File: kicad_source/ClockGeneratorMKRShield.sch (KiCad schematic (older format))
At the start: 3 parts, among them CN1 ARDUINO_MKR

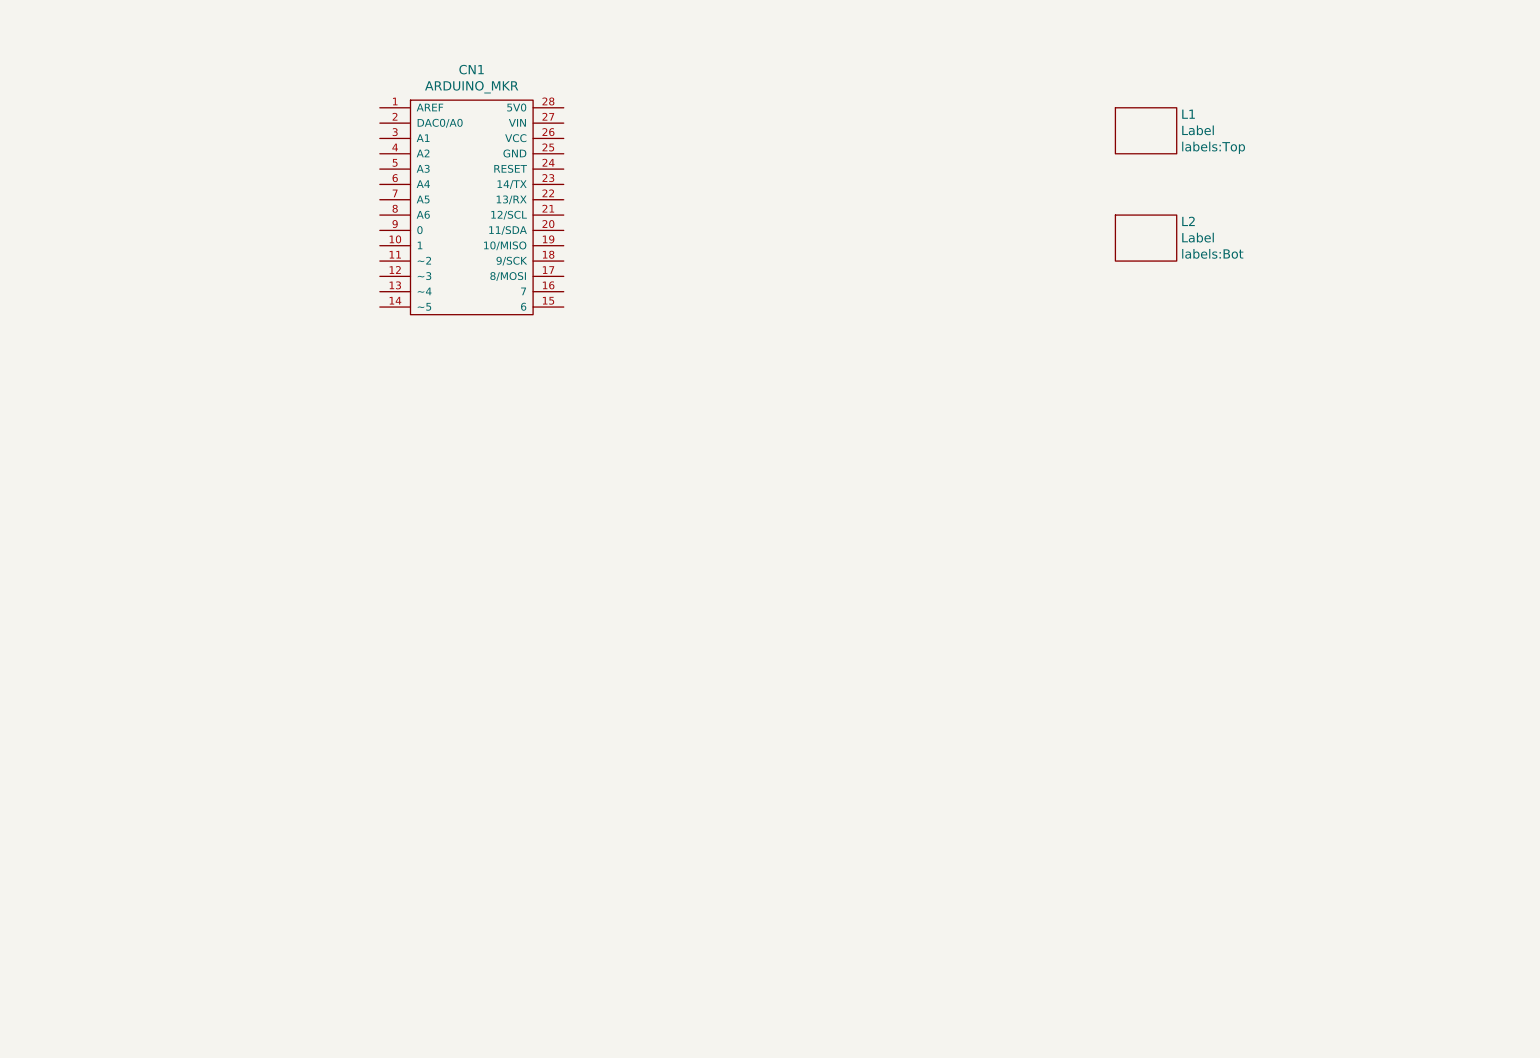
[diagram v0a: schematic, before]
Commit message: updated schematic
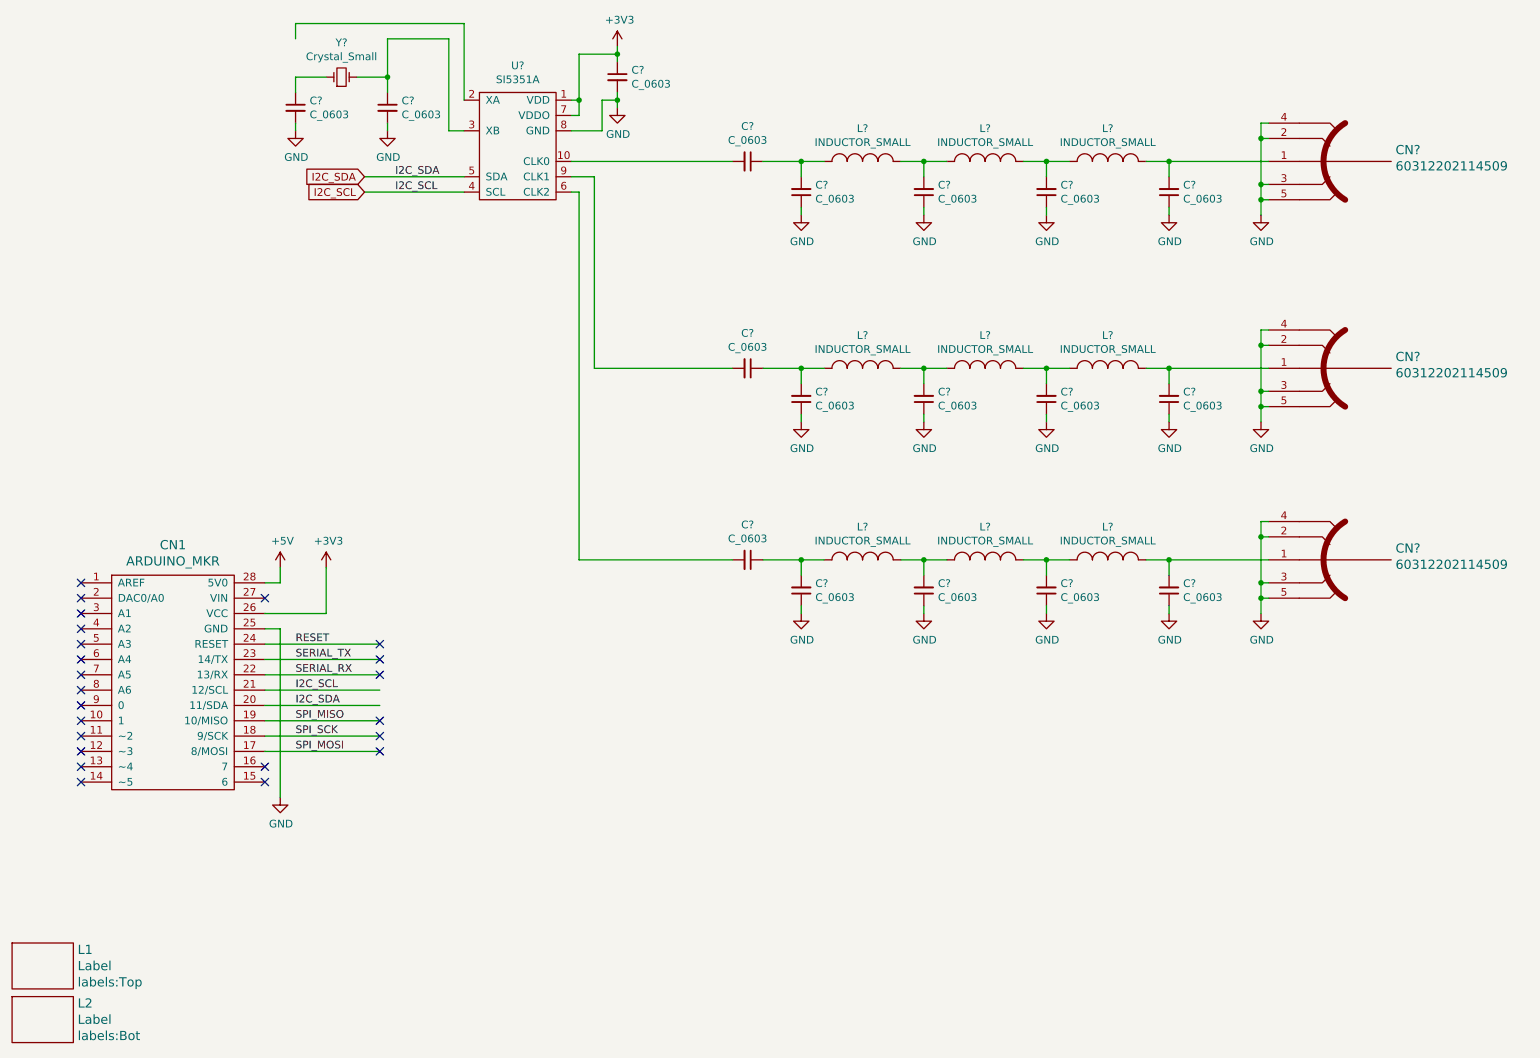
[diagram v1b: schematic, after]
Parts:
- added C? (x18): C_0603, capacitors:C_0603, symbol devices:C_0603
- added CN? (x3): 60312202114509, CON_wuerth:WR-SMA-PCB, symbol CON_wuerth:60312202114509
- added L? (x9): INDUCTOR_SMALL, L_filter:WE-CAIR_4248, symbol devices:INDUCTOR_SMALL
- added U?: SI5351A, SSOP:MSOP-10_3x3mm_Pitch0.5mm, symbol IC_interface_i2c:SI5351A
- added Y?: Crystal_Small, symbol devices:Crystal_Small
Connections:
- net SPI_MOSI: now reaches CN1.17 (8/MOSI)
- net SPI_SCK: now reaches CN1.18 (9/SCK)
- net SPI_MISO: now reaches CN1.19 (10/MISO)
- net I2C_SDA: now reaches CN1.20 (11/SDA)
- net I2C_SDA: now also U?.5 (SDA)
- net I2C_SCL: now reaches CN1.21 (12/SCL)
- net I2C_SCL: now also U?.4 (SCL)
- net SERIAL_RX: now reaches CN1.22 (13/RX)
- net SERIAL_TX: now reaches CN1.23 (14/TX)
- net RESET: now reaches CN1.24 (RESET)
- net GND: now reaches CN1.25 (GND)
- net GND: now also C?.1, C?.1, C?.1, C?.1, C?.1, C?.1, C?.1, C?.1, C?.1, C?.1, C?.1, C?.1, C?.2, C?.2, C?.2, CN?.2, CN?.2, CN?.2, CN?.3, CN?.3, CN?.3, CN?.4, CN?.4, CN?.4, CN?.5, CN?.5, CN?.5, U?.8 (GND)
- net +3V3: now reaches CN1.26 (VCC)
- net +3V3: now also C?.1, U?.1 (VDD), U?.7 (VDDO)
- net +5V: now reaches CN1.28 (5V0)
- new net: C?.2, U?.10 (CLK0)
- new net: C?.1, U?.3 (XB), Y?.2
- new net: C?.2, U?.6 (CLK2)
- new net: C?.2, U?.9 (CLK1)
- new net: C?.1, Y?.1
- new net: C?.1, C?.2, L?.1 (x3)
- new net: C?.2, L?.1, L?.2 (x6)
- new net: C?.2, CN?.1, L?.2 (x3)
- no-connect marks 0 -> 23
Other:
- moved on the sheet: CN1, L1, L2
